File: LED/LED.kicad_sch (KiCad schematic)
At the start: 25 parts, among them J1 USB_C_Receptacle_USB2.0, J2 RJ45, J3 RJ45, J4 Screw_Terminal_01x03, U1 CH340C, U2 WeMos_D1_mini, U3 ESP32-WROOM-32D, U4 AMS1117-3.3

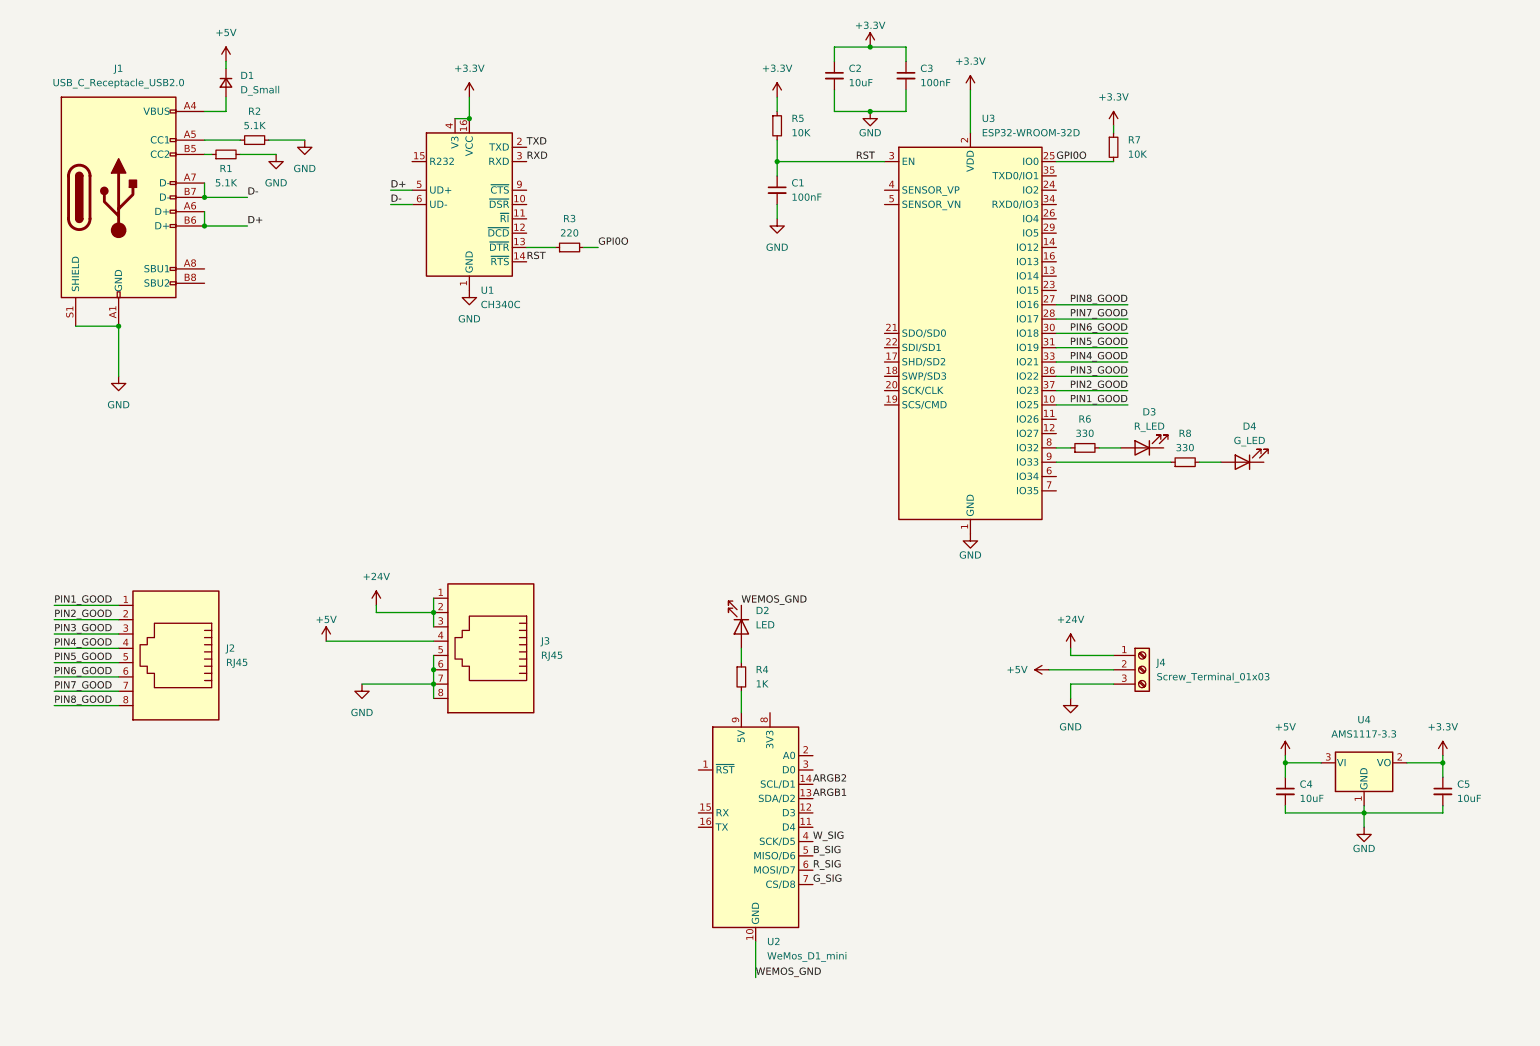
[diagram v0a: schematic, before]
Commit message: 2 ethernet
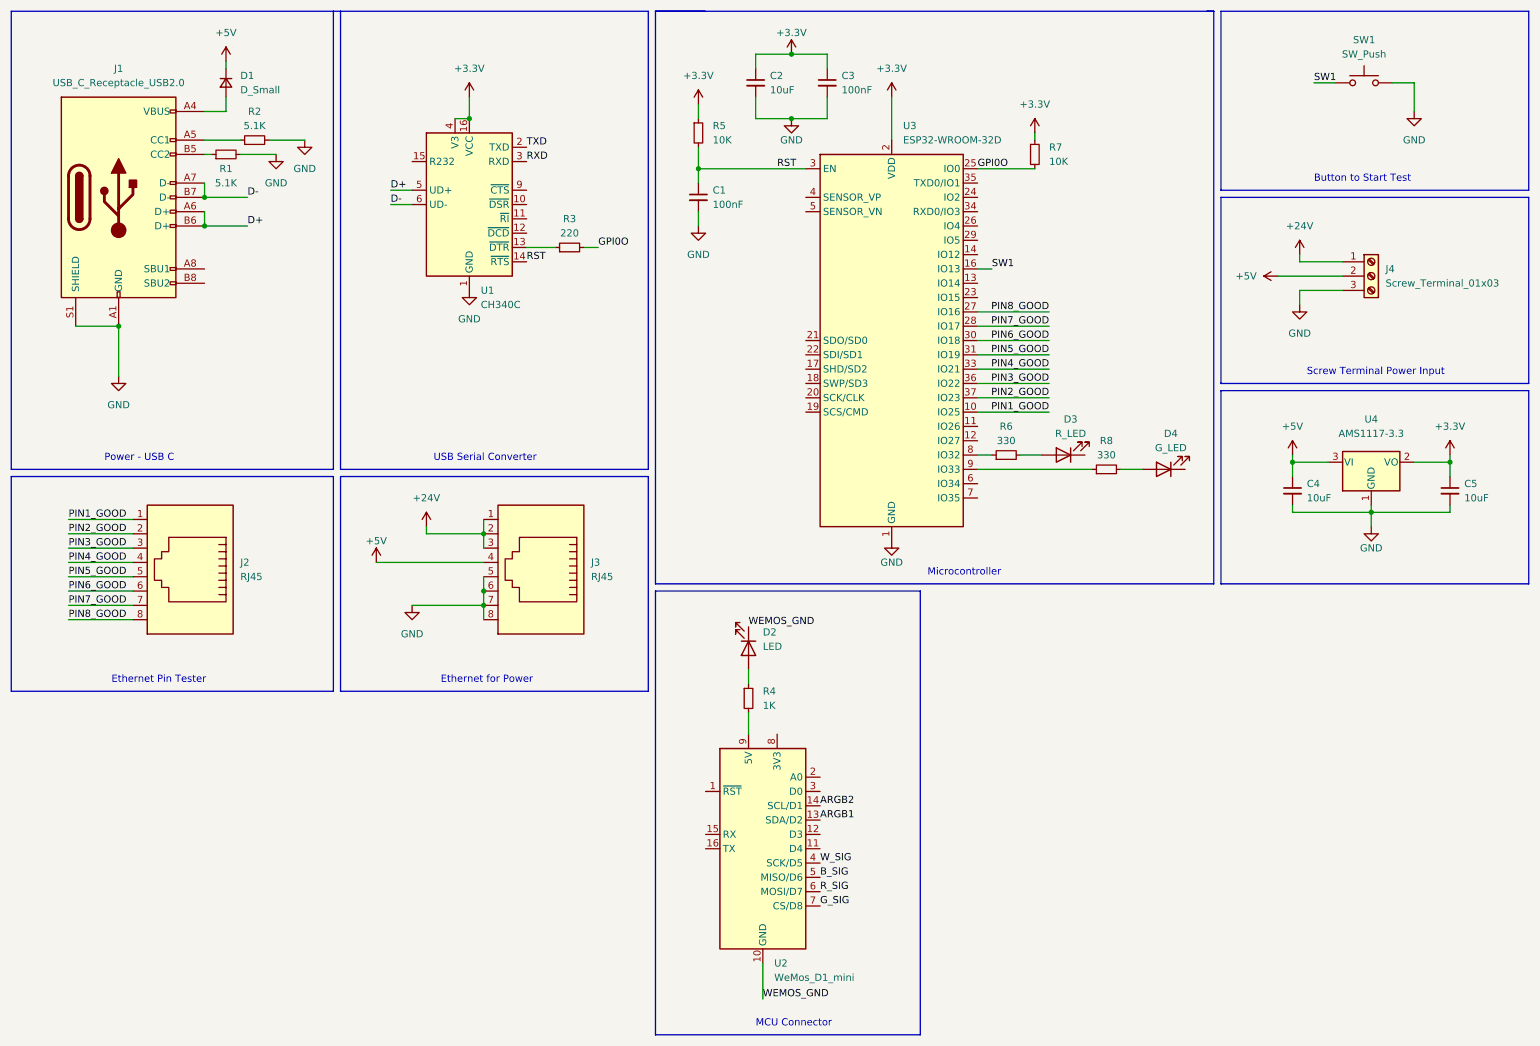
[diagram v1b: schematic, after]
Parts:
- added SW1: SW_Push, Button_Switch_THT:SW_PUSH_6mm, symbol Switch:SW_Push
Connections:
- net GND: now also SW1.2
- net SW1: now reaches U3.16 (IO13)
- net SW1: now also SW1.1
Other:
- note added: "Button to Start Test"
- note added: "Ethernet Pin Tester"
- note added: "Ethernet for Power"
- note added: "MCU Connector"
- note added: "Microcontroller"
- note added: "Power - USB C"
- note added: "Screw Terminal Power Input"
- note added: "USB Serial Converter"
- moved on the sheet: C1, C2, C3, C4, C5, D2, D3, D4, J2, J3, J4, R4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
